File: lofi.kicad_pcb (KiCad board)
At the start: 2 copper layers, 22 x 25.4 mm, 18 parts, among them J1 NRF24l01+, J2 ISP, J3 debug, SW1 Reed, U1 TPL5111, U2 MCP1711-3.3, U3 ATtiny84V

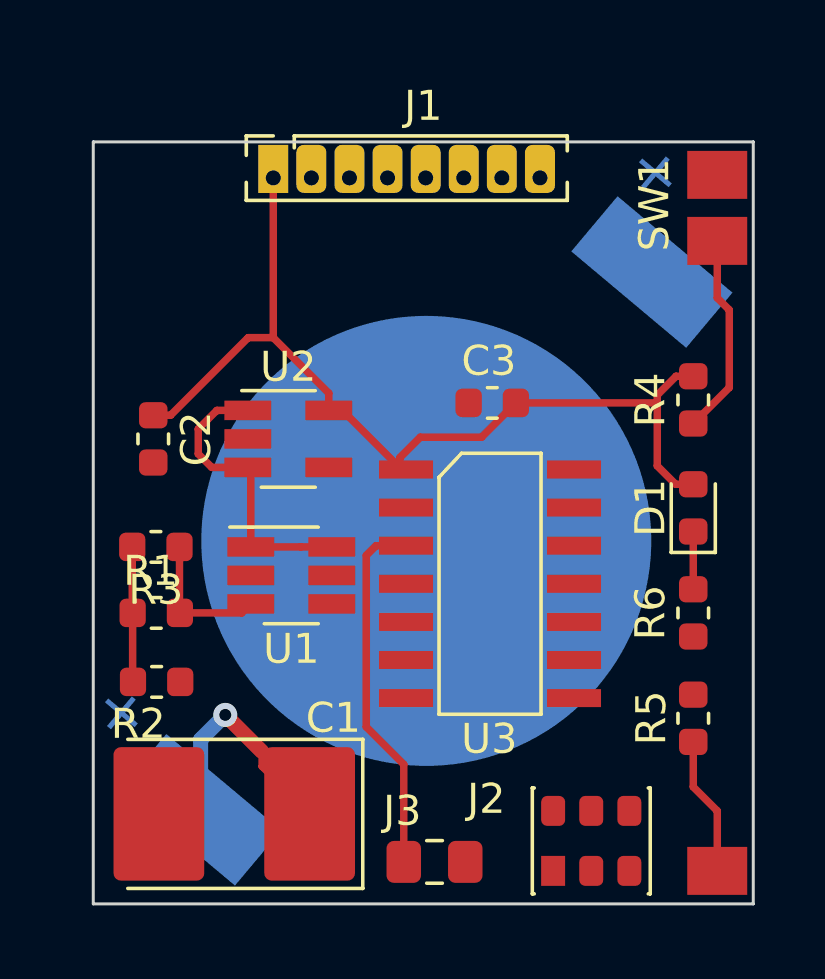
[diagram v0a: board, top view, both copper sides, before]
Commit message: as sent to OSHPark
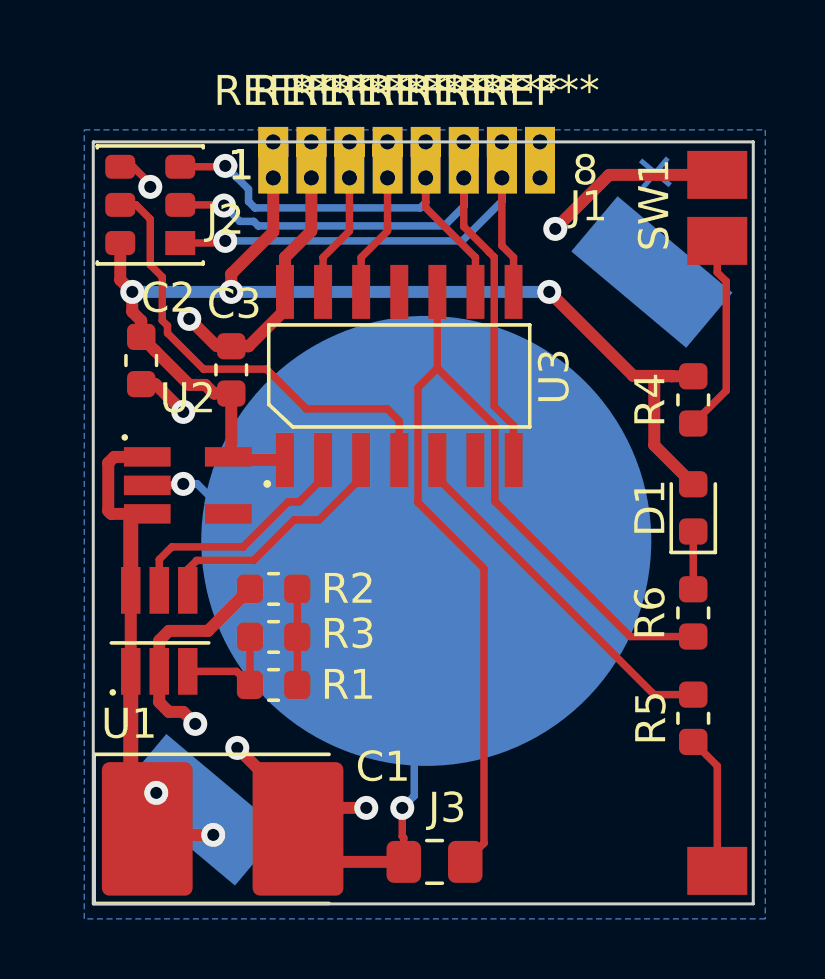
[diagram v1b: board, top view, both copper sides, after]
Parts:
- added REF**: castellate, lofi:castellate, F.Cu at (125.1, 69.2)
- added REF**: castellate, lofi:castellate, F.Cu at (123.8, 69.2)
- added REF**: castellate, lofi:castellate, F.Cu at (122.5, 69.2)
- added REF**: castellate, lofi:castellate, F.Cu at (121.3, 69.2)
- added REF**: castellate, lofi:castellate, F.Cu at (120.0, 69.2)
- added REF**: castellate, lofi:castellate, F.Cu at (118.7, 69.2)
- added REF**: castellate, lofi:castellate, F.Cu at (117.5, 69.2)
- added REF**: castellate, lofi:castellate, F.Cu at (116.2, 69.2)
- U1: footprint Package_TO_SOT_SMD:SOT-23-6_Handsoldering -> lofi:TPL5111
- U2: footprint Package_TO_SOT_SMD:SOT-23-5_HandSoldering -> lofi:MCP1711
- moved J2 25.8 mm to (112.1, 71.3), turned to 180 degrees
- moved C3 8.77 mm to (114.8, 76.8), turned to 90 degrees
- moved U3 7.56 mm to (120.4, 77.0), turned to 90 degrees
- moved R2 4.98 mm to (116.2, 84.1), turned to 180 degrees
- moved R3 4.94 mm to (116.2, 85.7), turned to 0 degrees
- moved U1 4.77 mm to (112.4, 85.5), turned to 90 degrees
- moved R1 4.59 mm to (116.2, 87.3), turned to 0 degrees
- moved U2 3.69 mm to (113.3, 80.7)
- moved C2 2.64 mm to (111.8, 76.5)
- moved C1 0.63 mm to (114.5, 92.1), turned to 0 degrees
- turned J3 to 180 degrees
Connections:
- net Net-(J1-Pad3) renamed /CE
- net Net-(J1-Pad4) renamed /CSN
- net Net-(J1-Pad7) renamed /MISO
- J1 pad 5: Net-(J1-Pad5) -> /SCK
- J1 pad 6: Net-(J1-Pad6) -> /MOSI
- J2 pad 3: Net-(J1-Pad5) -> /MOSI
- J2 pad 4: Net-(J1-Pad6) -> /RSTn
- J2 pad 5: Net-(J2-Pad5) -> /SCK
- U3 pad 10: Net-(U1-Pad4) -> Net-(J3-Pad1)
- U3 pad 11: Net-(U1-Pad5) -> Net-(U3-Pad11)
- U3 pad 2: Net-(U3-Pad2) -> Net-(U1-Pad5)
- U3 pad 3: Net-(J3-Pad1) -> Net-(U1-Pad4)
- U3 pad 4: Net-(J2-Pad5) -> /RSTn
- U3 pad 7: Net-(J1-Pad6) -> /MOSI
- U3 pad 9: Net-(J1-Pad5) -> /SCK
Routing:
- net GND: track 0.00 -> 58.4 mm, vias 0 -> 9
- net Net-(J3-Pad1): track 12.0 -> 34.1 mm
- net /MOSI: track 0.00 -> 21.0 mm, vias 0 -> 1
- net /MISO: track 0.00 -> 16.0 mm, vias 0 -> 1
- net /RSTn: track 0.00 -> 15.5 mm
- net /SCK: track 0.00 -> 14.7 mm, vias 0 -> 1
- net Net-(R5-Pad1): track 0.00 -> 12.1 mm
- net +3V3: track 31.8 -> 40.7 mm, vias 0 -> 3
- net Net-(U1-Pad4): track 0.00 -> 8.34 mm
- net Net-(U1-Pad5): track 0.00 -> 8.22 mm
- net /CSN: track 0.00 -> 4.16 mm
- net /CE: track 0.00 -> 4.16 mm
- net Net-(R1-Pad2): track 4.51 -> 3.20 mm
- net Net-(R1-Pad1): track 4.69 -> 3.86 mm
- net Net-(R4-Pad1): track 6.10 -> 6.67 mm
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- added copper zone on B.Cu, net GND
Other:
- board text added: "lofi ver 0.1"
